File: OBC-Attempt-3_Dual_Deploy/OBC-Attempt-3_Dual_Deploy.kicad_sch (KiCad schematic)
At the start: 29 parts, among them J1 Bat, J2 Bat, J3 PWR, J4 DEBUG, J5 CAN Header, J6 Conn_01x02_Female, J7 Conn_01x02_Female, SW1 SW_SPDT, SW2 SW_SPST, U1 LD1117S33TR_SOT223, U2 STM32F042G4Ux, U3 SN65HVD230, U4 CPC1002N, U5 CPC1002N, X1 ECS-2520MV-xxx-xx

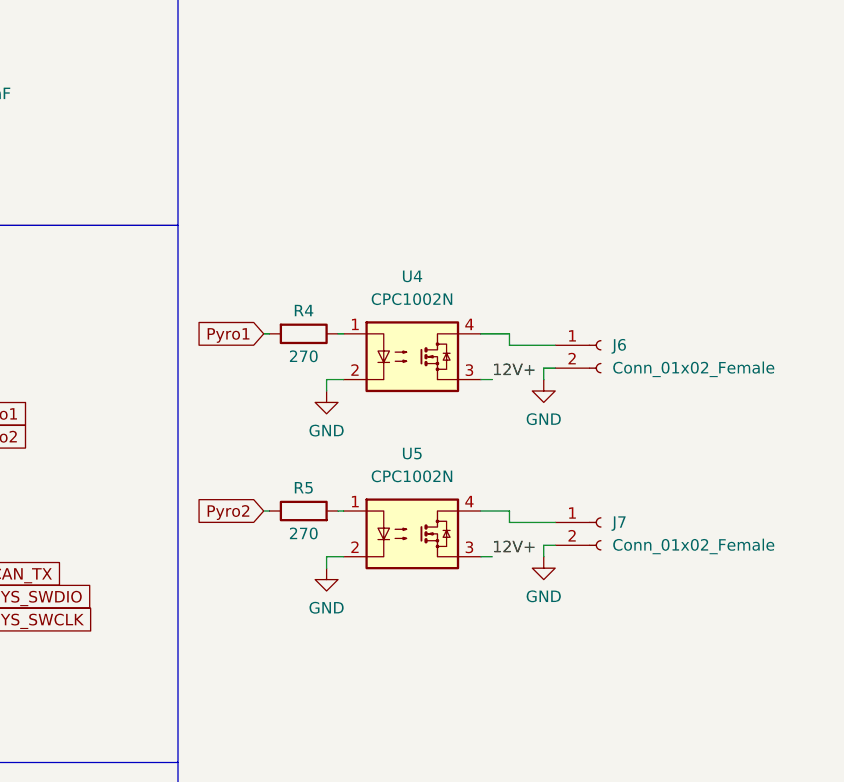
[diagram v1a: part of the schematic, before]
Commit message: Cherry Rework
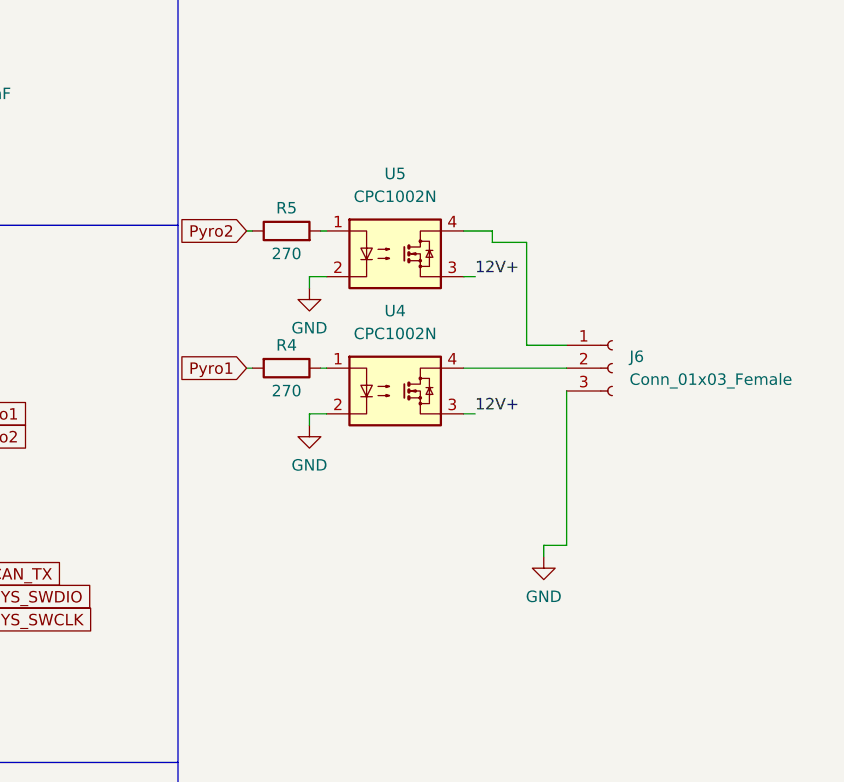
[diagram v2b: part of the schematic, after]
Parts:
- removed J6, J7: Conn_01x02_Female, Connector_PinHeader_1.00mm:PinHeader_1x02_P1.00mm_Vertical, symbol Connector:Conn_01x02_Female
- added J6: Conn_01x03_Female, Connector_PinSocket_2.54mm:PinSocket_1x03_P2.54mm_Vertical, symbol Connector:Conn_01x03_Female
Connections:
- net GND: now also J6.3 (Pin_3)
- net at U5.4: now also J6.1 (Pin_1)
- net at U4.4: now also J6.2 (Pin_2)
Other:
- moved on the sheet: R4, R5, U4, U5
